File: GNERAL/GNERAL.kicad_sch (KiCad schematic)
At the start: 6 parts

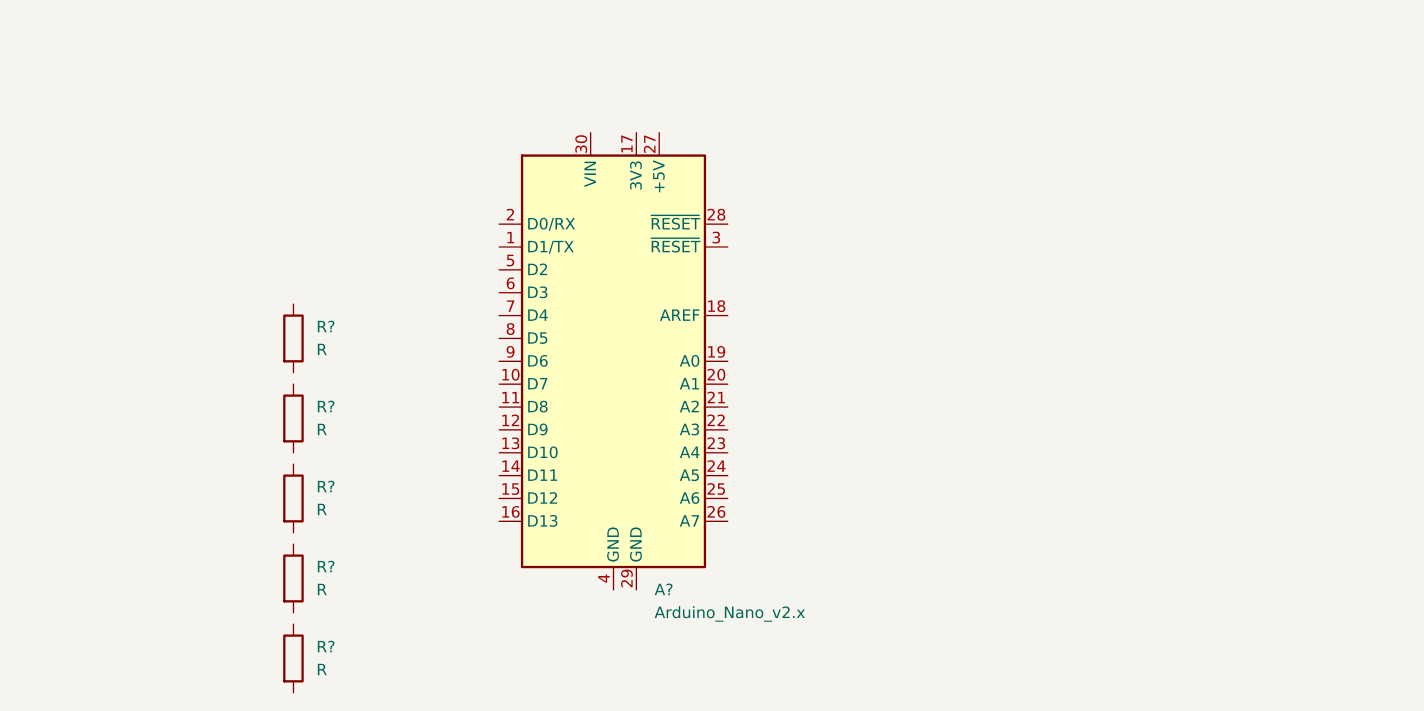
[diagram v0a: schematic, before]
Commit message: medio
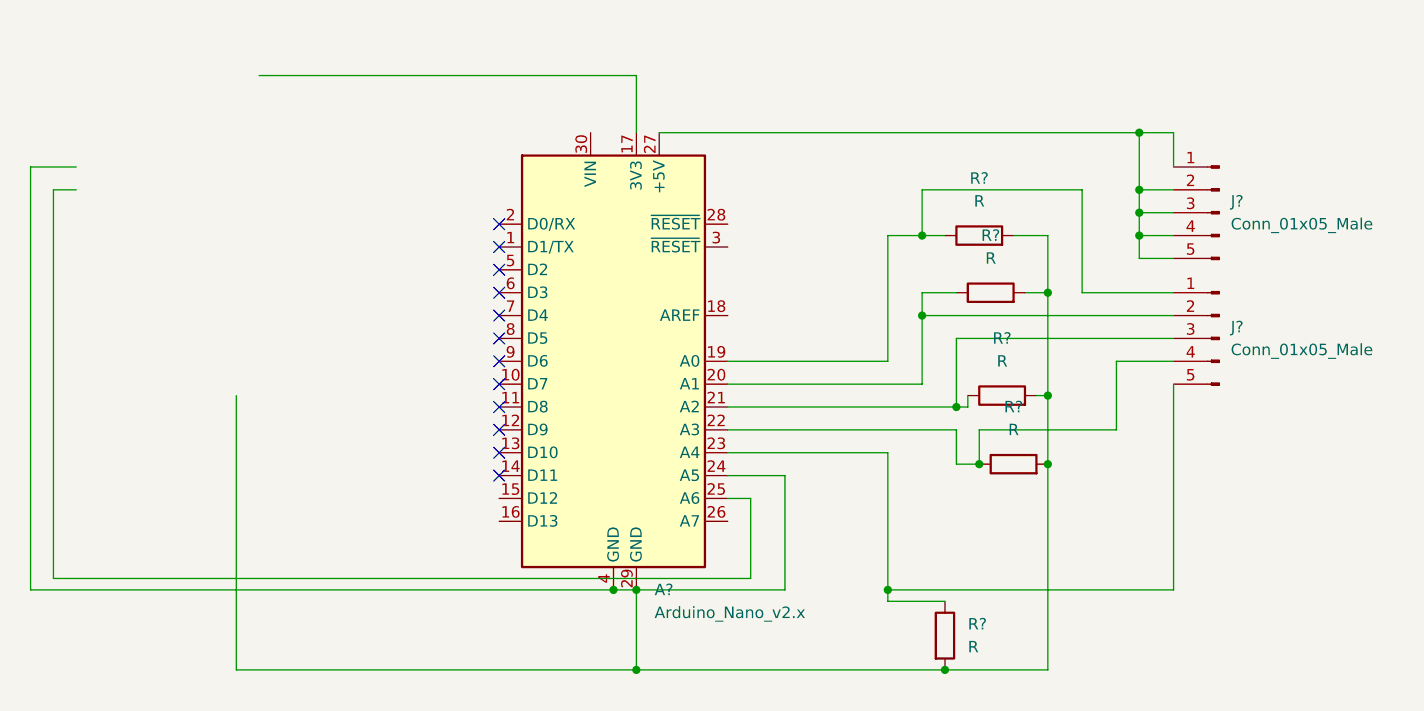
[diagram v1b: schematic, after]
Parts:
- added J?: Conn_01x05_Male, Connector_JST:JST_XH_B5B-XH-A_1x05_P2.50mm_Vertical, symbol Connector:Conn_01x05_Male
- added J?: Conn_01x05_Male, symbol Connector:Conn_01x05_Male
- R?: footprint (none) -> Resistor_SMD:R_0805_2012Metric_Pad1.20x1.40mm_HandSolder
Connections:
- net at R?.1: now also A?.21 (A2), J?.3 (Pin_3)
- net at R?.2: now also A?.24 (A5), A?.29 (GND), A?.4 (GND), R?.2, R?.2, R?.2, R?.2
- net at R?.1: now also A?.19 (A0), J?.1 (Pin_1)
- net at R?.1: now also A?.20 (A1), J?.2 (Pin_2)
- net at A?.22 (A3): now also R?.1, J?.4 (Pin_4)
- net at A?.23 (A4): now also R?.1, J?.5 (Pin_5)
- net at A?.27 (+5V): now also J?.1 (Pin_1), J?.2 (Pin_2), J?.3 (Pin_3), J?.4 (Pin_4), J?.5 (Pin_5)
- no-connect marks 0 -> 12
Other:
- moved on the sheet: R?

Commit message: hola
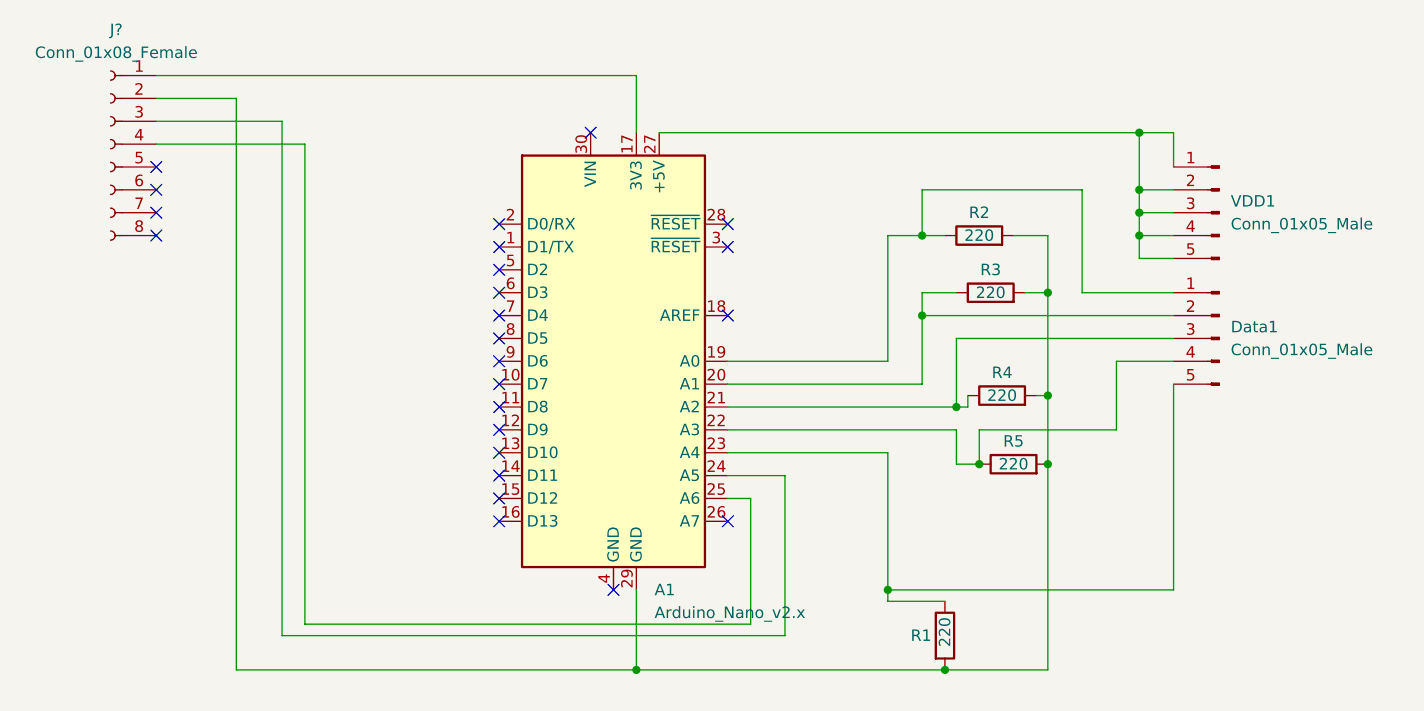
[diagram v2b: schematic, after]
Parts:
- added J?: Conn_01x08_Female, Connector_PinSocket_2.54mm:PinSocket_1x08_P2.54mm_Vertical, symbol Connector:Conn_01x08_Female
- R1, R2, R3, R4, R5: renamed from R?; value R -> 220
- VDD1: renamed from J?; footprint (none) -> Connector_JST:JST_XH_B5B-XH-A_1x05_P2.50mm_Vertical
- gave numbers to parts that had none: 2
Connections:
- net at A1.29 (GND), R1.2, R2.2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: now also J?.2 (Pin_2); no longer A1.24 (A5), A1.4 (GND)
- net at A1.17 (3V3): now also J?.1 (Pin_1)
- net at A1.25 (A6): now also J?.4 (Pin_4)
- new net: A1.24 (A5), J?.3 (Pin_3)
- no-connect marks 12 -> 24
